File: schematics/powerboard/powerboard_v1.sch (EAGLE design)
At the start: 20 parts, among them IC1 ACS756LCB-100B-PFF-T, IC2 AD2302ARDZ-5

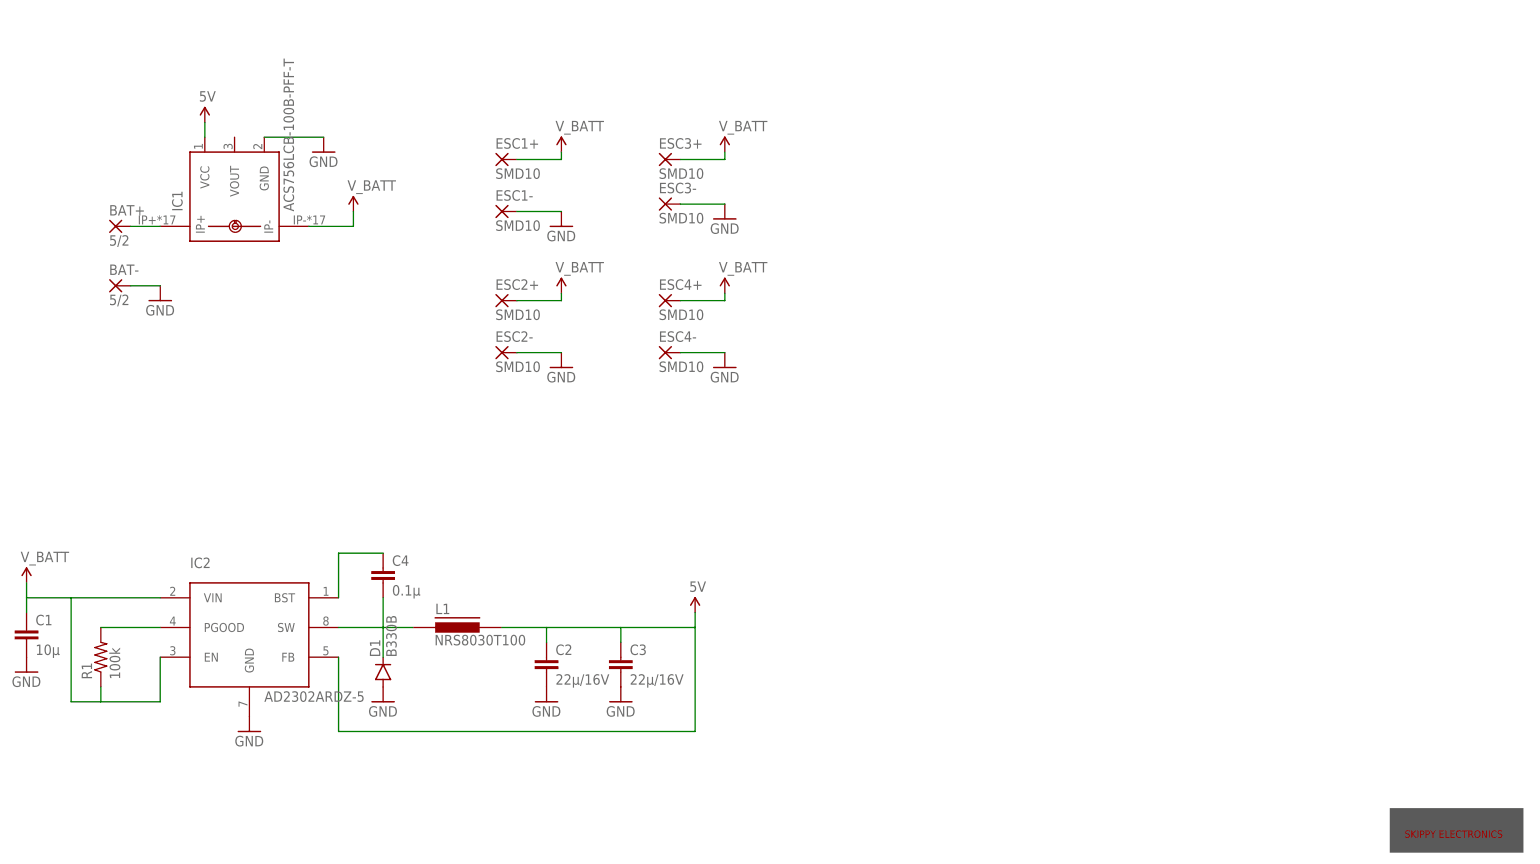
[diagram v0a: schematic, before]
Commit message: Power board finalized
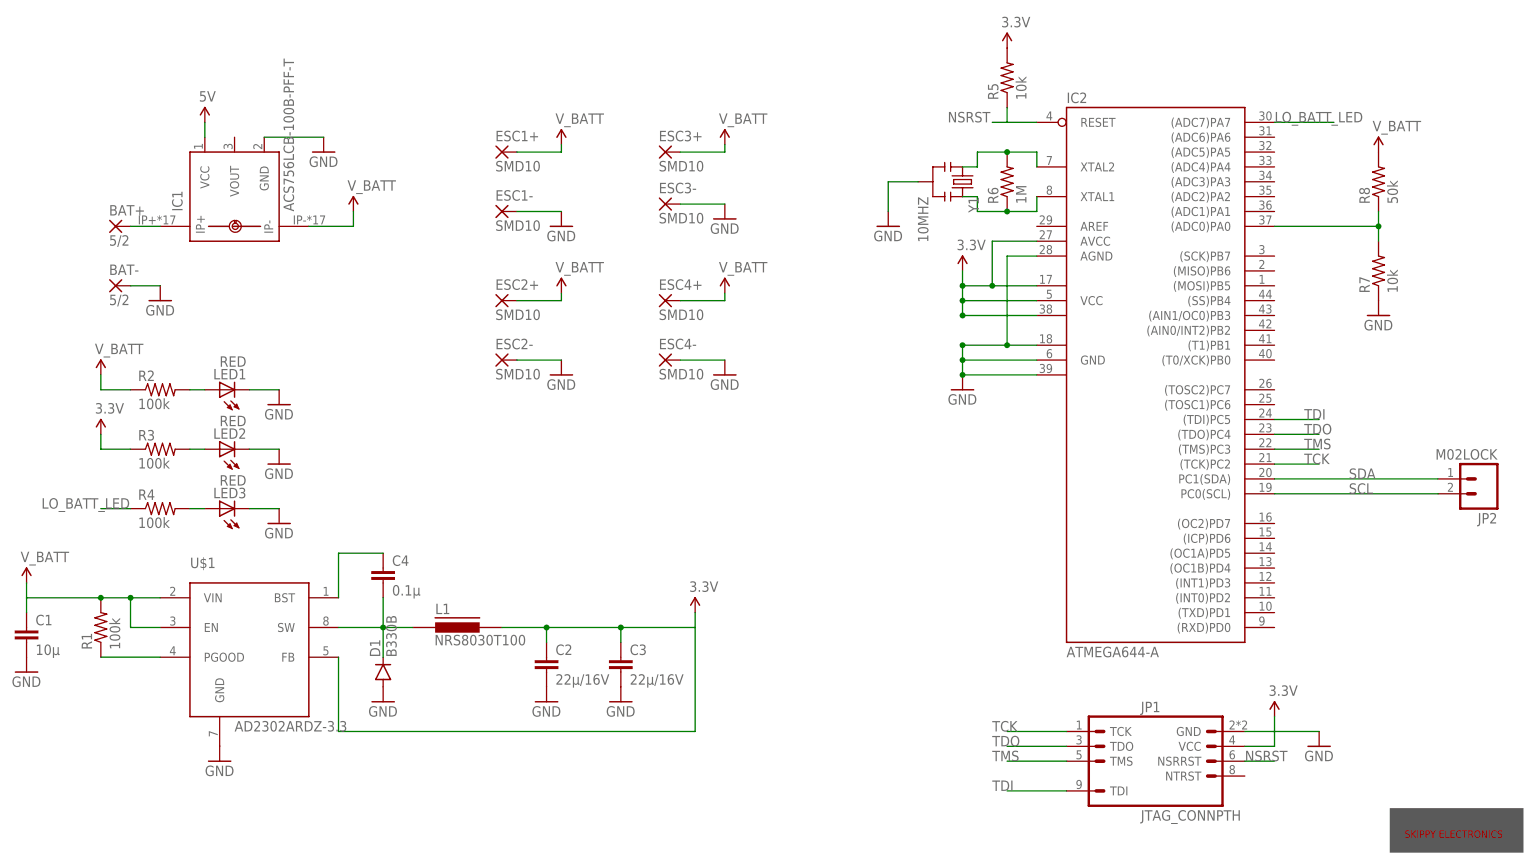
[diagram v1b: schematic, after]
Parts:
- added JP1: JTAG_CONNPTH, connectors:JTAG_CONNPTH
- added JP2: M02LOCK, SparkFun-Connectors:M02LOCK
- added LED1, LED2, LED3: RED, eagle-ltspice:LED_E
- added R2, R3, R4: 100k, SparkFun-Passives:RESISTOR1206
- added R5, R7: 10k, SparkFun-Passives:RESISTOR1206
- added R6: 1M, SparkFun-Passives:RESISTOR1206
- added R8: 50k, SparkFun-Passives:RESISTOR1206
- added U$1: AD2302ARDZ-3.3, dcdcconv:AD2302ARDZ-3.3
- added Y1: 10MHZ, SparkFun-FreqCtrl:RESONATOR8MHZ
- IC2: value AD2302ARDZ-5 -> ATMEGA644-A; device dcdcconv:AD2302ARDZ-5 -> atmega:ATMEGA644-A
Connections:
- new net 3.3V: C2.1, C3.1, IC2.AVCC, IC2.VCC, IC2.VCC1, IC2.VCC2, JP1.VCC, L1.2, R3.1, R5.2, U$1.FB
- new net LO_BATT_LED: IC2.(ADC7)PA7, R4.1
- new net N$10: IC2.(ADC0)PA0, R7.2, R8.1
- new net N$3: R1.1, U$1.PGOOD
- new net N$4: LED1.A, R2.2
- new net N$7: LED3.A, R4.2
- new net N$8: IC2.XTAL2, R6.2, Y1.1
- new net N$9: IC2.XTAL1, R6.1, Y1.3
- new net NSRST: IC2.RESET, JP1.NSRRST, R5.1
- new net SCL: IC2.PC0(SCL), JP2.2
- new net SDA: IC2.PC1(SDA), JP2.1
- new net TCK: IC2.(TCK)PC2, JP1.TCK
- new net TDI: IC2.(TDI)PC5, JP1.TDI
- new net TDO: IC2.(TDO)PC4, JP1.TDO
- new net TMS: IC2.(TMS)PC3, JP1.TMS
- net 5V: no longer C2.1, C3.1, IC2.FB, L1.2
- net GND: now also IC2.AGND, IC2.GND1, IC2.GND2, JP1.GND, LED1.C, LED2.C, LED3.C, R7.1, U$1.GND, Y1.2
- net N$2: now also U$1.SW; no longer IC2.SW
- net N$5: now also U$1.BST; no longer IC2.BST
- net N$6: now also LED2.A, R3.2; no longer IC2.PGOOD, R1.2
- net V_BATT: now also R1.2, R2.1, R8.2, U$1.EN, U$1.VIN; no longer IC2.EN, IC2.VIN, R1.1
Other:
- moved on the sheet: ESC1+, ESC2-, ESC3+, ESC4-, R1
